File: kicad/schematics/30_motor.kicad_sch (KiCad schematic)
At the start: 0 parts

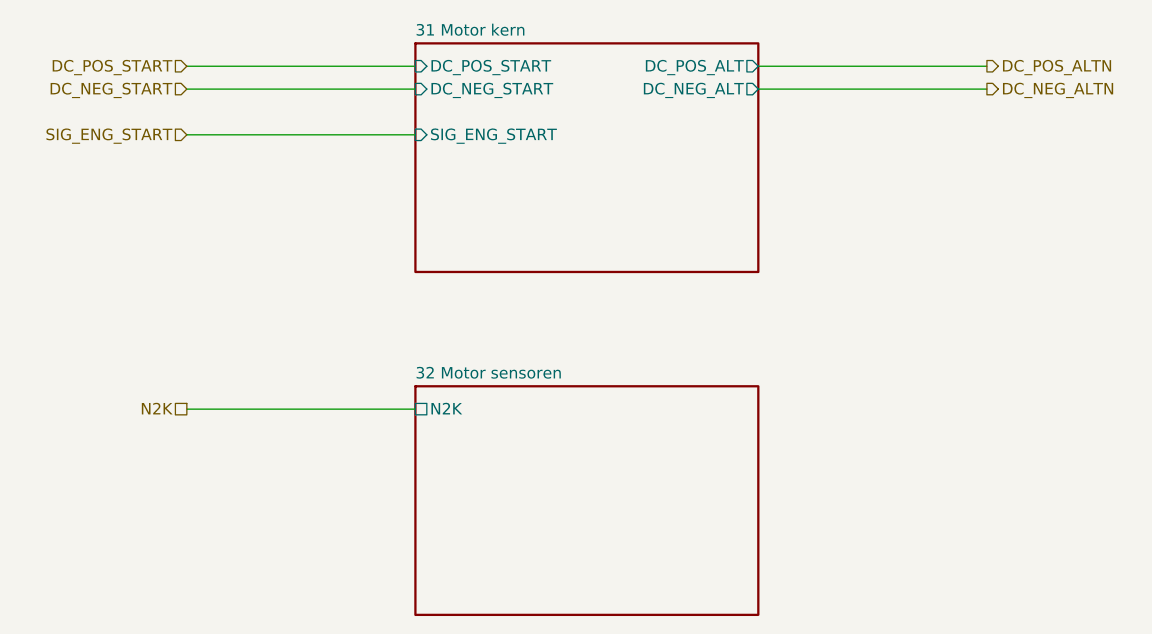
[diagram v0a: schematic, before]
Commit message: eerste opzet 21_laden_opslag_distributie
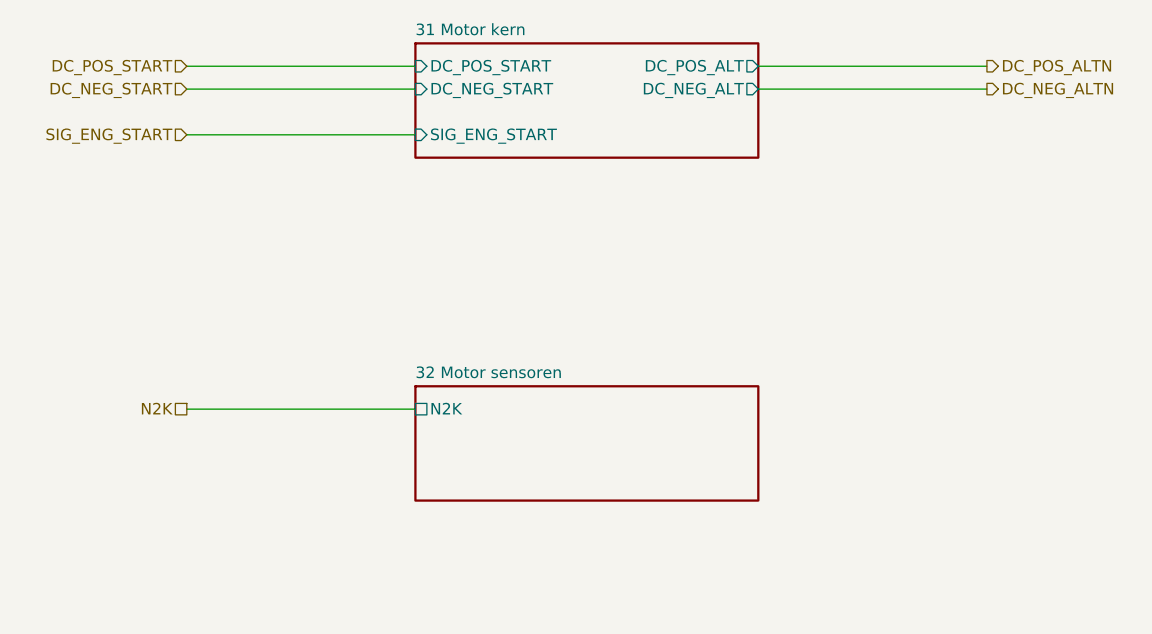
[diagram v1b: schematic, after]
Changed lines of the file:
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@@
 	(sheet
 		(at 88.9 63.5)
-		(size 38.1 25.4)
+		(size 38.1 12.7)
 		(exclude_from_sim no)
 		(in_bom yes)
@@
 		)
 		(property "Sheetname" "32 Motor sensoren"
-			(at 88.9 62.7884 0)
+			(at 88.9 62.7376 0)
 			(show_name no)
 			(do_not_autoplace no)
@@
 		)
 		(property "Sheetfile" "32_motor_sensoren.kicad_sch"
-			(at 88.9 89.4846 0)
+			(at 88.9 76.8354 0)
 			(hide yes)
 			(show_name no)
@@
 	(sheet
 		(at 88.9 25.4)
-		(size 38.1 25.4)
+		(size 38.1 12.7)
 		(exclude_from_sim no)
 		(in_bom yes)
@@
 		)
 		(property "Sheetname" "31 Motor kern"
-			(at 88.9 24.6884 0)
+			(at 88.9 24.6376 0)
 			(show_name no)
 			(do_not_autoplace no)
@@
 		)
 		(property "Sheetfile" "31_motor_kern.kicad_sch"
-			(at 88.9 51.3846 0)
+			(at 88.9 38.7354 0)
 			(hide yes)
 			(show_name no)
